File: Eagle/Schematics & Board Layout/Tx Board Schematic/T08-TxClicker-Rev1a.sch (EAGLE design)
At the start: 83 parts, among them U1 CC430F513X---RGZ48, X1-DNI SMA-SMD, Y1 26MHz

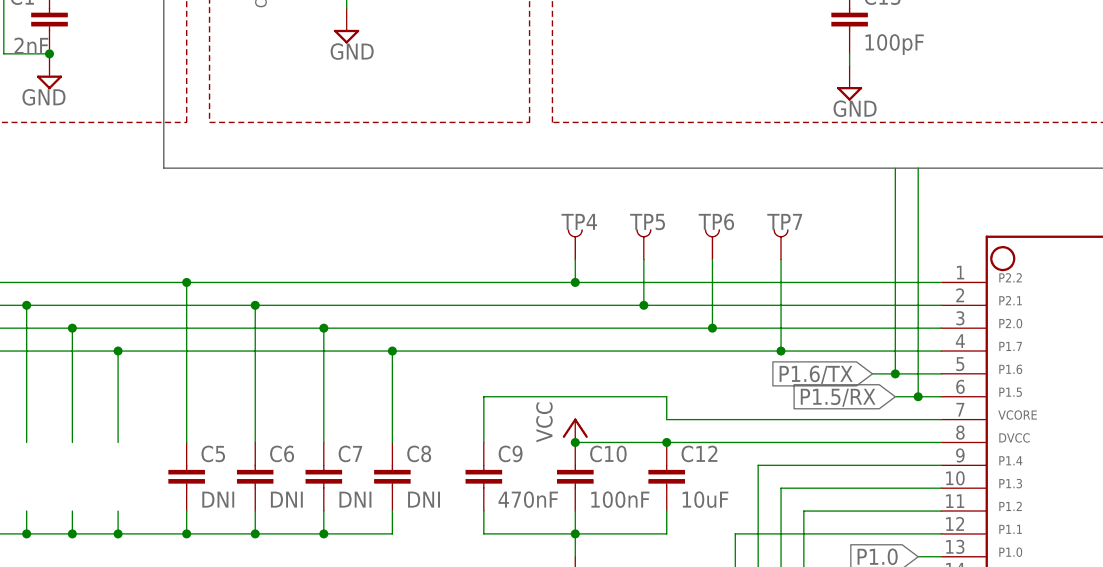
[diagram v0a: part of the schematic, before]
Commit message: layout update
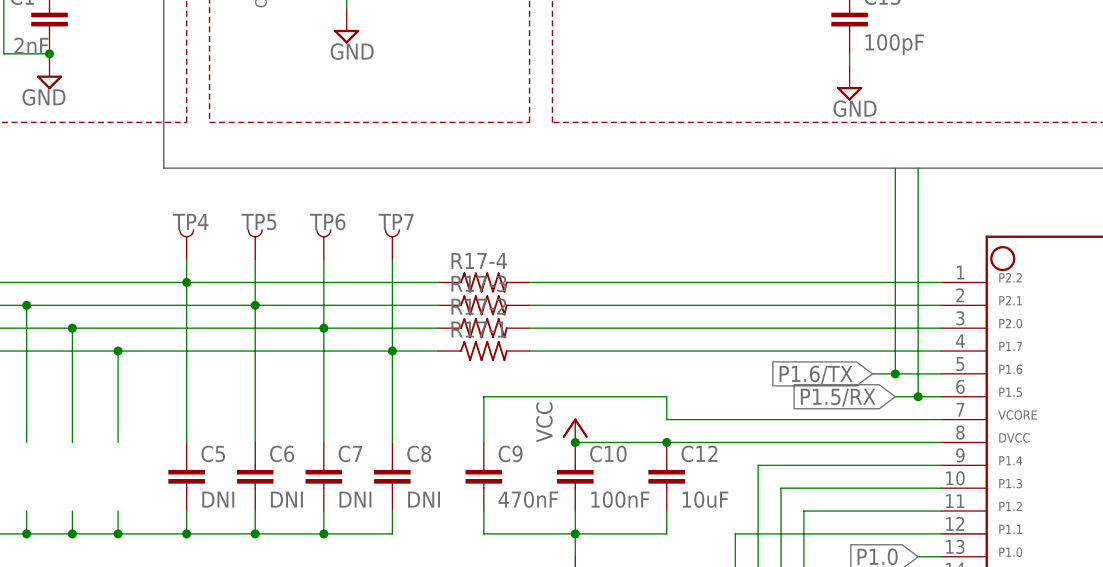
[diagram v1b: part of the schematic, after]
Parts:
- added R17: (no value), QuadResistor:R603X42012
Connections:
- new net N$19: R17-3.2, U1.2
- new net N$20: R17-4.2, U1.1
- new net N$7: R17-1.2, U1.4
- new net N$9: R17-2.2, U1.3
- net P1.7: now also R17-1.1; no longer U1.4
- net P2.0: now also R17-2.1; no longer U1.3
- net P2.1: now also R17-3.1; no longer U1.2
- net P2.2: now also R17-4.1; no longer U1.1
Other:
- moved on the sheet: TP4, TP5, TP6, TP7
